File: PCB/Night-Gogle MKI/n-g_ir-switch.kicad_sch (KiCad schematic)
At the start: 4 parts, among them U1 IRL540N

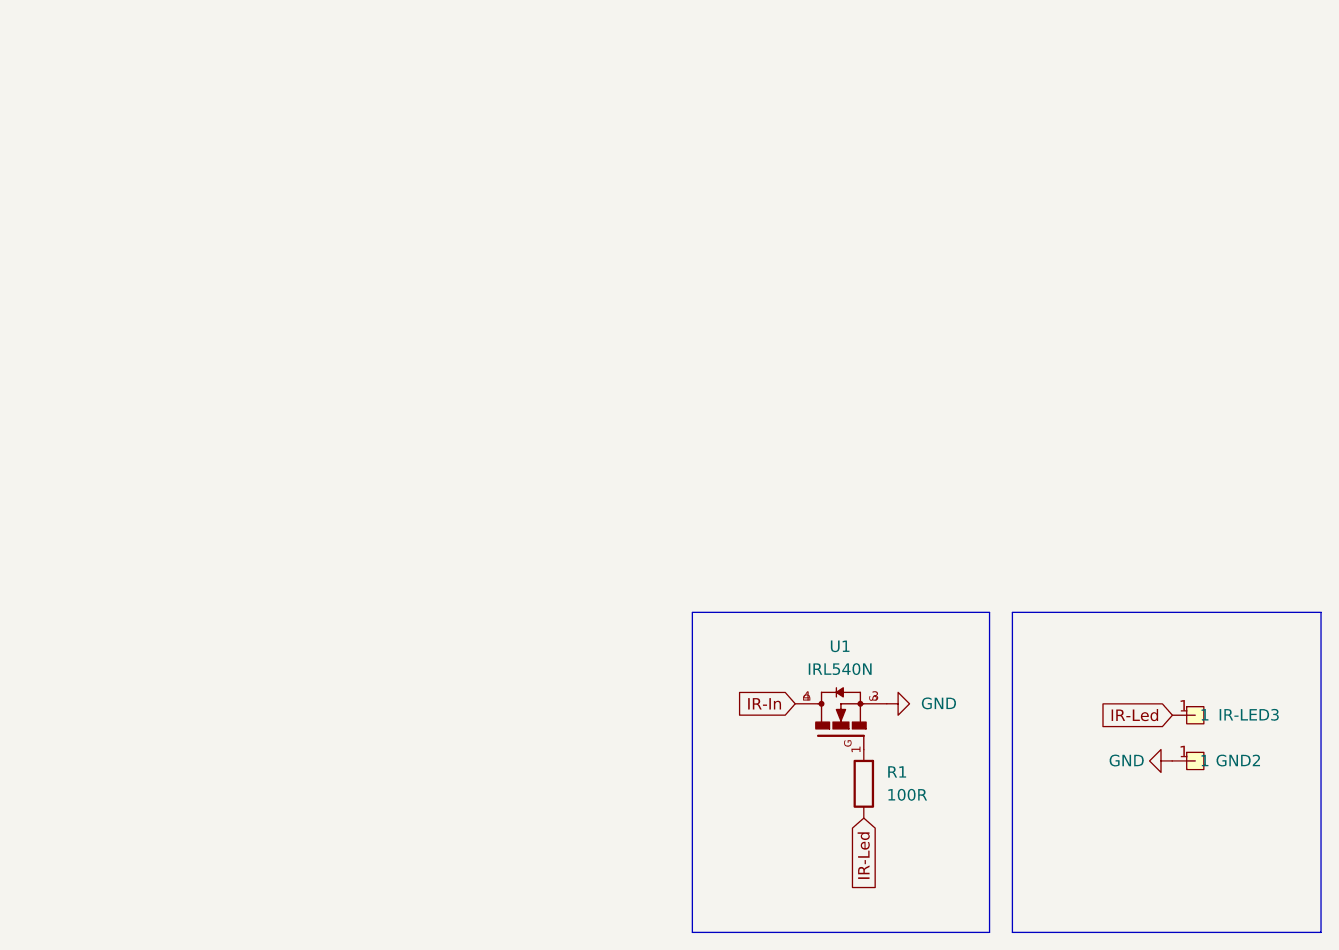
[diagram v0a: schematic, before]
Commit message: gg
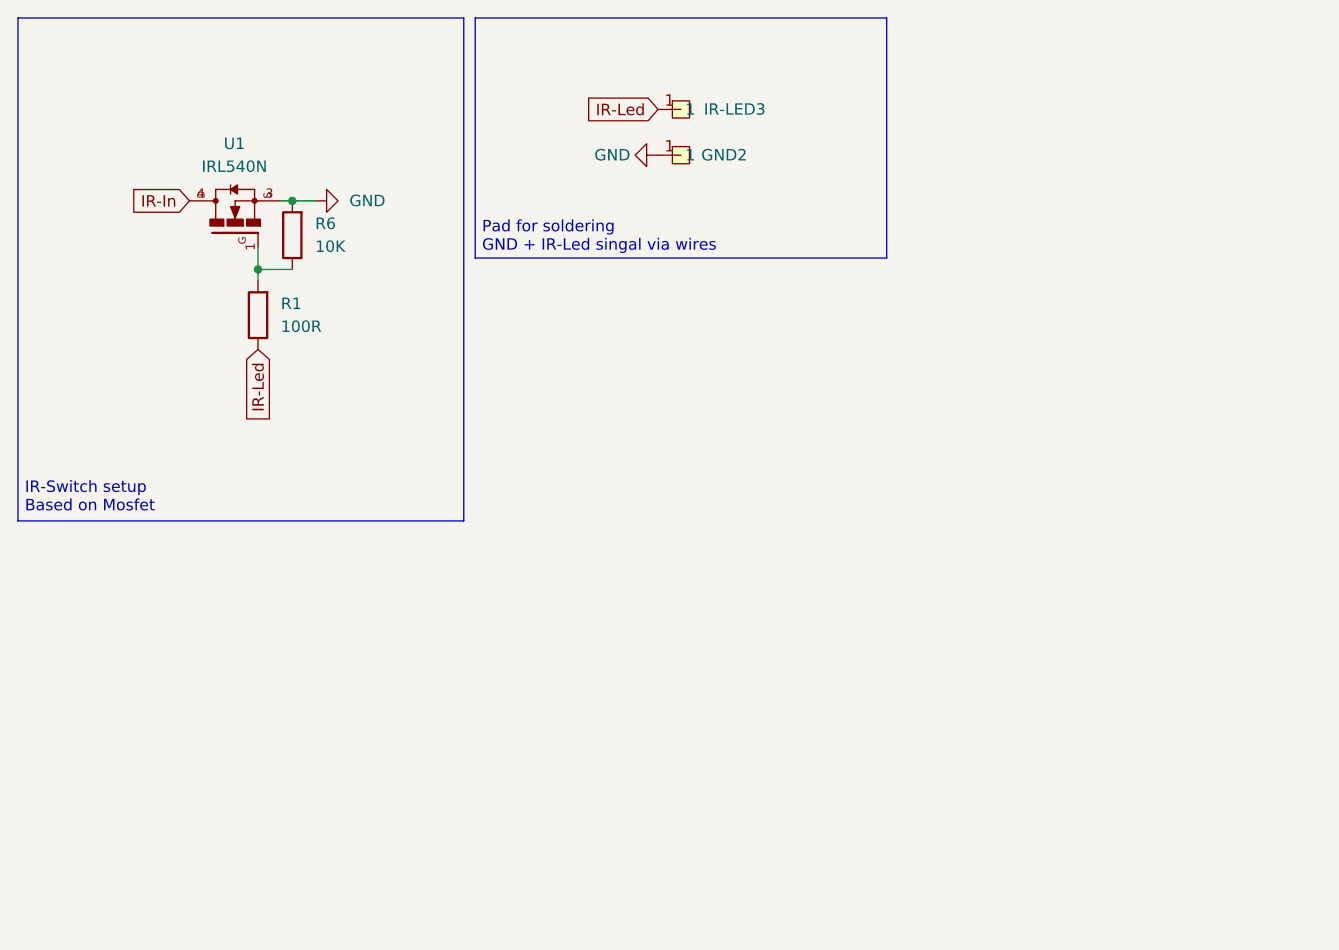
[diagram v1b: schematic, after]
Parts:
- added R6: 10K, Resistor_SMD:R_0805_2012Metric_Pad1.20x1.40mm_HandSolder, symbol Device:R
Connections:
- net GND: now also R6.2
- net at R1.2, U1.1: now also R6.1
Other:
- note added: "IR-Switch setup Based on Mosfet"
- note added: "Pad for soldering GND + IR-Led singal via wires"
- moved on the sheet: GND2, IR-LED3, R1, U1
